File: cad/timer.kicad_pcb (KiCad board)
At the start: 2 copper layers, 111.8 x 45.7 mm, 17 parts, among them J1 Motor, J2 Pot, Q1 S9012, Q2 S9013, Q3 S9012, U1 ATMEGA328P-PU, U2 LM393, U3 L293D, Y1 AB38T-32.768kHz

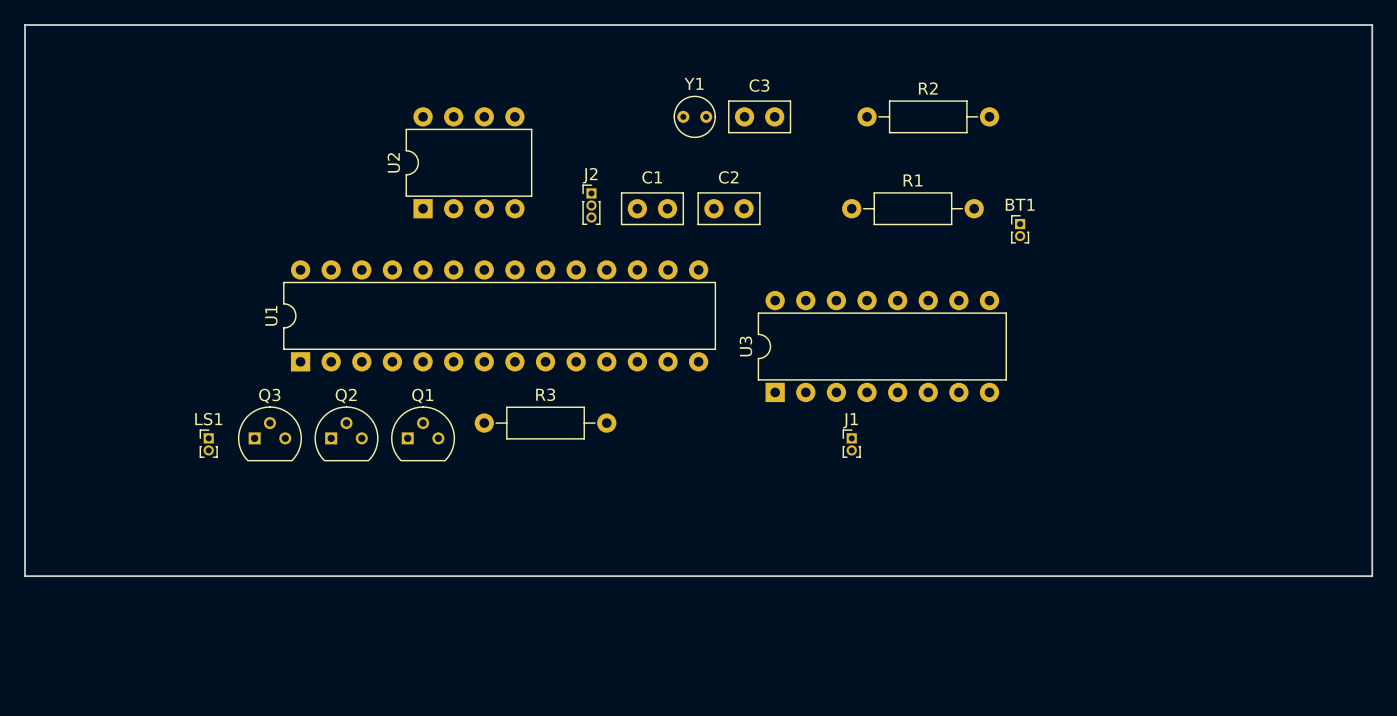
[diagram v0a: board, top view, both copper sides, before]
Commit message: CAD files for first PCB attempt
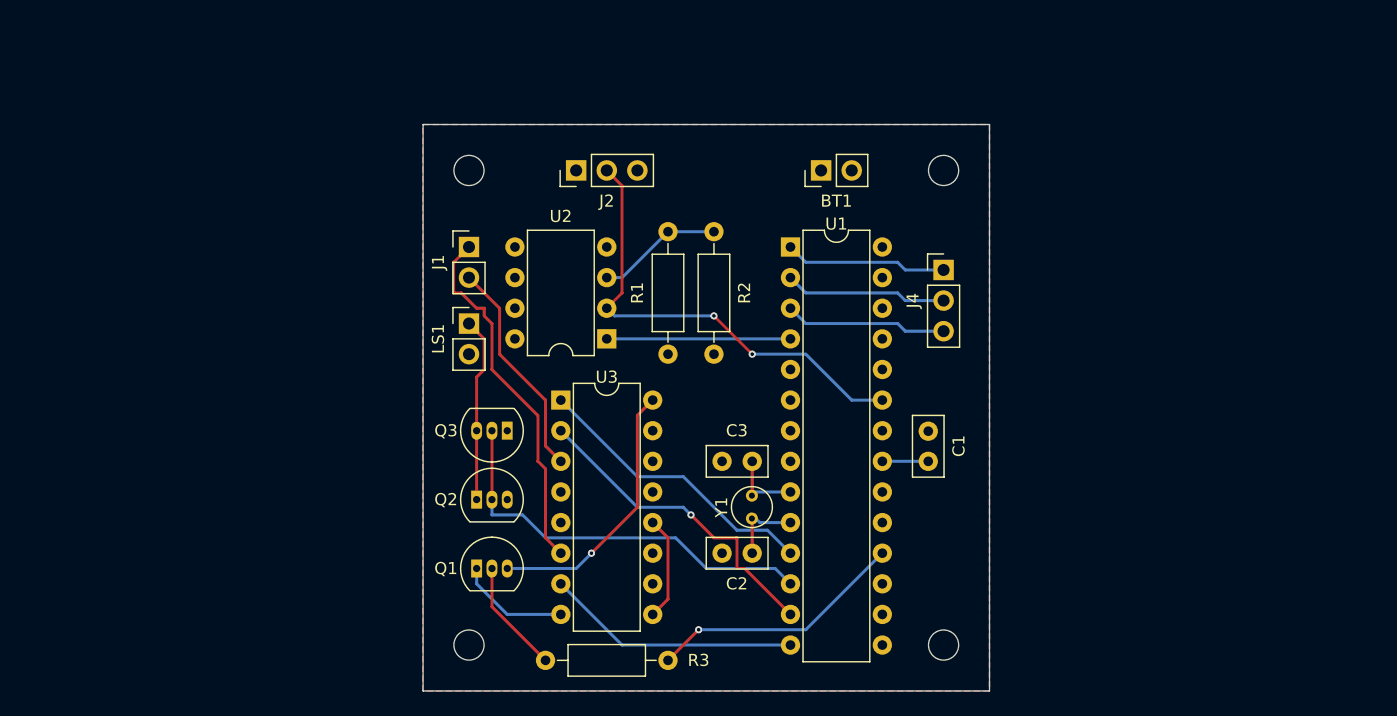
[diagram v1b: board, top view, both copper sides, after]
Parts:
- added H1: MountingHole_2.5mm, Mounting_Holes:MountingHole_2.5mm, F.Cu at (125.7, 73.0)
- added H2: MountingHole_2.5mm, Mounting_Holes:MountingHole_2.5mm, F.Cu at (165.1, 73.0)
- added H3: MountingHole_2.5mm, Mounting_Holes:MountingHole_2.5mm, F.Cu at (165.1, 112.4)
- added H4: MountingHole_2.5mm, Mounting_Holes:MountingHole_2.5mm, F.Cu at (125.7, 112.4)
- added J4: Prog, Pin_Headers:Pin_Header_Straight_1x03_Pitch2.54mm, F.Cu at (165.1, 81.3)
- BT1, J1: footprint Pin_Headers:Pin_Header_Straight_1x02_Pitch1.00mm -> Pin_Headers:Pin_Header_Straight_1x02_Pitch2.54mm
- C1: value 47p -> 47pF
- C2, C3: value 15p -> 15pF
- J2: footprint Pin_Headers:Pin_Header_Straight_1x03_Pitch1.00mm -> Pin_Headers:Pin_Header_Straight_1x03_Pitch2.54mm
- LS1: value PSR-36N08A-JQ -> Speaker; footprint Pin_Headers:Pin_Header_Straight_1x02_Pitch1.00mm -> Pin_Headers:Pin_Header_Straight_1x02_Pitch2.54mm
- Q1, Q2, Q3: footprint TO_SOT_Packages_THT:TO-92_Molded_Narrow -> TO_SOT_Packages_THT:TO-92_Inline_Narrow_Oval
- R1: value 1M -> 1MΩ
- R2: value 47k -> 47kΩ
- R3: value 10k -> 10kΩ
- Y1: value AB38T-32.768kHz -> 32.768kHz
- moved U1 41.7 mm to (152.4, 79.4), turned to 0 degrees
- moved J1 35.5 mm to (125.7, 79.4)
- moved Y1 33.8 mm to (149.2, 101.9), turned to 90 degrees
- moved C1 32.0 mm to (163.8, 97.2), turned to 90 degrees
- moved C2 28.8 mm to (149.2, 104.8), turned to 180 degrees
- moved C3 28.6 mm to (149.2, 97.2), turned to 180 degrees
- moved LS1 23.6 mm to (125.7, 85.7)
- moved R3 20.3 mm to (132.1, 113.7)
- moved Q3 19.1 mm to (126.4, 100.3)
- moved U2 18.7 mm to (137.2, 87.0), turned to 180 degrees
- moved U3 17.8 mm to (133.3, 92.1), turned to 0 degrees
- moved BT1 17.1 mm to (154.9, 73.0), turned to 90 degrees
- moved R2 15.9 mm to (146.1, 78.1), turned to 270 degrees
- moved R1 15.4 mm to (142.2, 78.1), turned to 270 degrees
- moved Q2 14.6 mm to (128.9, 94.6), turned to 180 degrees
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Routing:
- net Net-(J2-Pad2): track 0.00 -> 38.5 mm, vias 0 -> 2
- net Net-(Q2-Pad2): track 0.00 -> 34.1 mm
- net Net-(J1-Pad1): track 0.00 -> 30.4 mm
- net Net-(U1-Pad13): track 0.00 -> 26.9 mm, vias 0 -> 1
- net Net-(U1-Pad11): track 0.00 -> 24.3 mm
- net Net-(Q1-Pad3): track 0.00 -> 22.3 mm, vias 0 -> 1
- net Net-(R3-Pad2): track 0.00 -> 21.5 mm, vias 0 -> 1
- net Net-(U1-Pad14): track 0.00 -> 21.2 mm
- net Net-(J1-Pad2): track 0.00 -> 18.4 mm
- net Net-(LS1-Pad1): track 0.00 -> 15.4 mm
- net Net-(U1-Pad4): track 0.00 -> 15.2 mm
- net Net-(J4-Pad3): track 0.00 -> 13.5 mm
- net Net-(J4-Pad1): track 0.00 -> 13.5 mm
- net Net-(J4-Pad2): track 0.00 -> 13.5 mm
- net Net-(R1-Pad1): track 0.00 -> 10.5 mm
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- added copper zone on B.Cu, net GND
- added copper zone on F.Cu, net VCC
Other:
- board size 111.8 x 45.7 mm -> 47 x 47 mm
- rule trace_min: 0.2 -> 0.1778
- rule via_min_size: 0.4 -> 0.381
